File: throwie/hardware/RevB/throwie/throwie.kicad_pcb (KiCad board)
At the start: 2 copper layers, 24 parts, among them J1 CONN, Q1 2SC3356, Q2 SS8050-G, T1 TestPoints, T2 TestPoints, T3 TestPoints, T4 TestPoints, U1 C8051F850-A-GU, U2 MIC5231-3.3YM5-TR, X1 RO3101

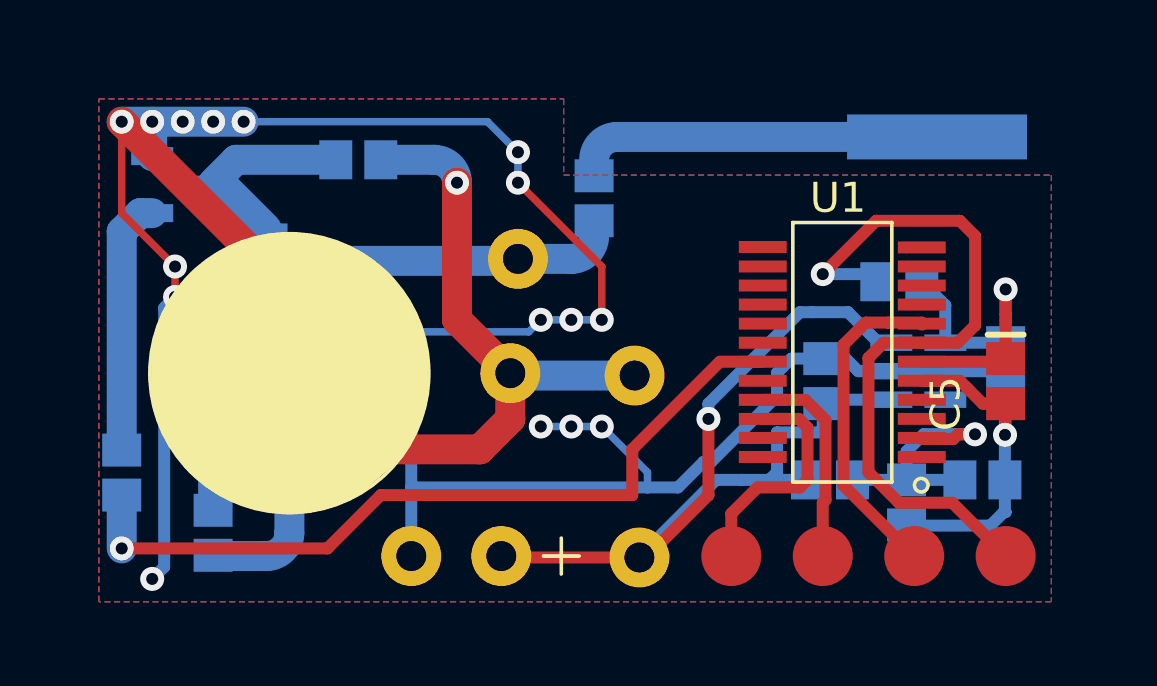
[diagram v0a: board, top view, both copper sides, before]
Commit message: final layout
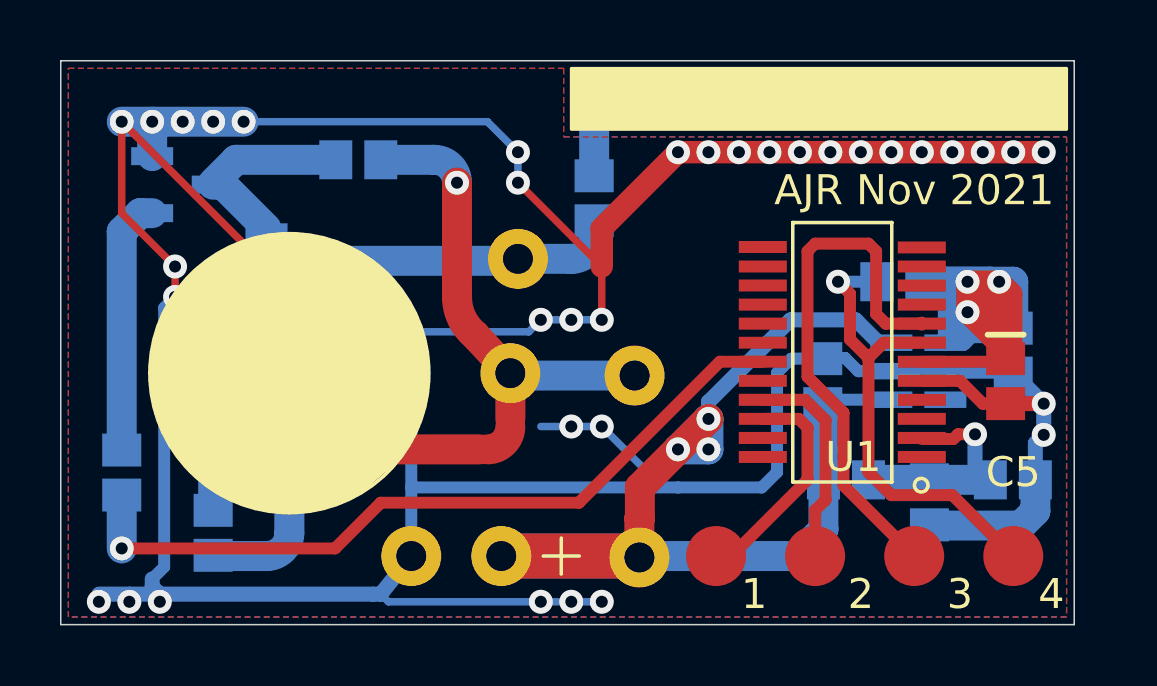
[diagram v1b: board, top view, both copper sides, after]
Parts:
- moved A1 1.98 mm to (51.1, 145.5)
- moved R3 1.02 mm to (51.6, 158.5)
- moved C6 0.76 mm to (49.5, 158.5)
- moved C2 0.55 mm to (52.3, 153.4)
- moved R2 0.53 mm to (46.0, 158.5)
- moved T1 0.51 mm to (42.4, 161.0)
- moved T2 0.25 mm to (45.7, 161.0)
- moved T3 0.25 mm to (52.3, 161.0)
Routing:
- net GNDREF: track 106.0 -> 145.4 mm, vias 18 -> 36
- net +3V3: track 11.3 -> 37.5 mm, vias 1 -> 3
- net +BATT: track 34.0 -> 43.2 mm, vias 1 -> 3
- net Net-(R5-Pad2): track 24.4 -> 16.4 mm
- net Net-(T4-Pad1): track 11.0 -> 17.9 mm
- net Net-(A1-Pad1): track 12.7 -> 15.5 mm
- net /0.471: track 8.89 -> 7.79 mm
- net /MOD: track 28.4 -> 27.5 mm
- net Net-(C4-Pad1): track 29.6 -> 30.2 mm
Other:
- board outline added: 33.8 x 18.8 mm
- board text added: "1"
- board text added: "2"
- board text added: "3"
- board text added: "4"
- board text added: "AJR Nov 2021"
